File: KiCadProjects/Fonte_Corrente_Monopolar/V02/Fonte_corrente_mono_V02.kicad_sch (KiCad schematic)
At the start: 33 parts, among them J1 alimentacao analogica, J2 sinais analogicos, J3 comunicacao / sinais digitais, J4 signal select, J7 +3.3V | +5.0V, U1-howland1 AD828AN, U2-INA-I1 INA128, U3-cond1 AD828AN

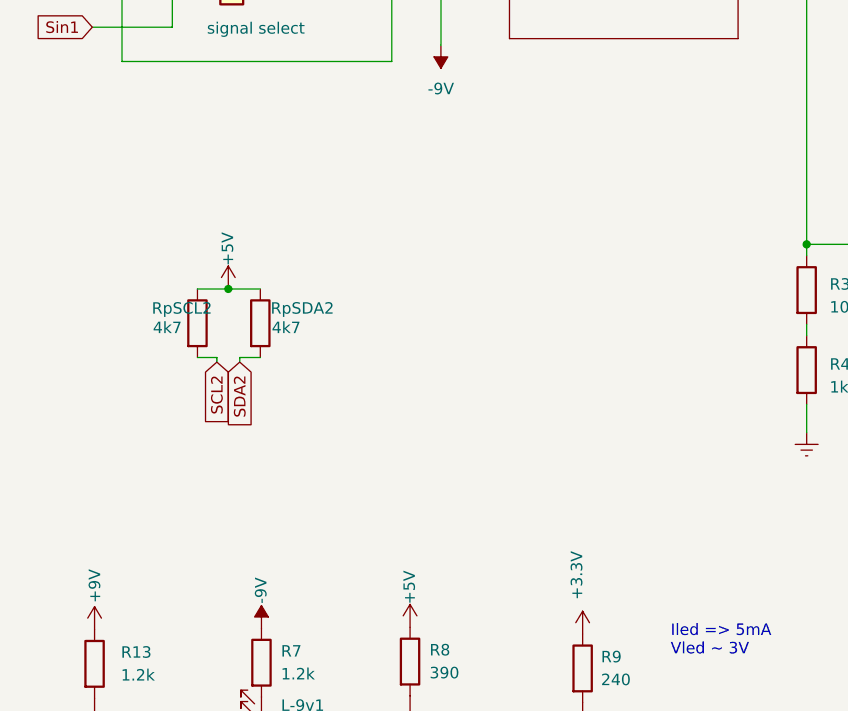
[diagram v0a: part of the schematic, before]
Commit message: temp
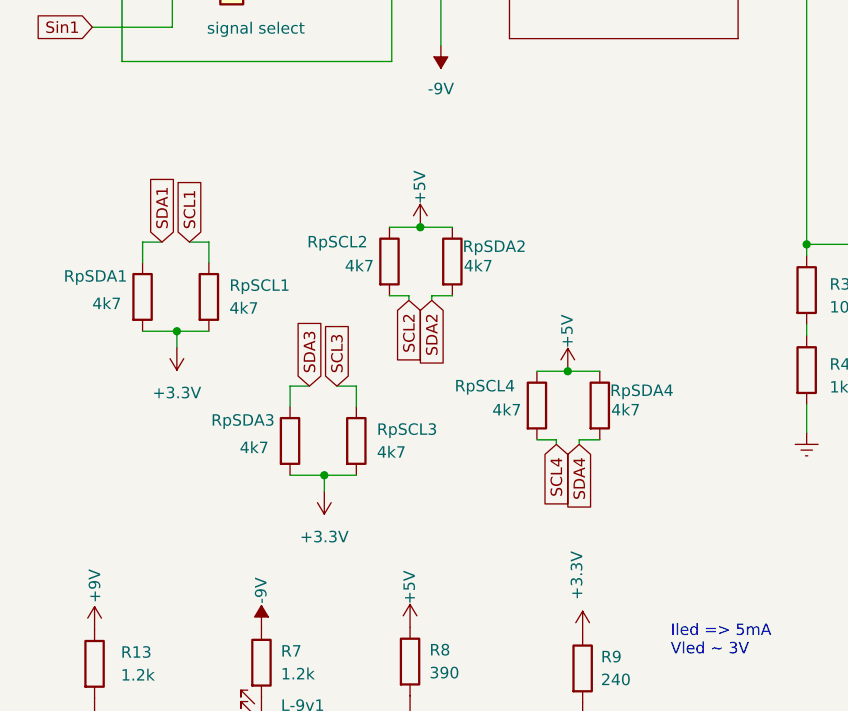
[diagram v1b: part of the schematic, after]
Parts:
- added RpSCL1, RpSCL3, RpSCL4, RpSDA1, RpSDA3, RpSDA4: 4k7, Resistor_THT:R_Axial_DIN0207_L6.3mm_D2.5mm_P7.62mm_Horizontal, symbol Device:R
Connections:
- net +3.3V: now also RpSCL1.2, RpSCL3.2, RpSDA1.2, RpSDA3.2
- net +5V: now also RpSCL4.1, RpSDA4.1
- net SCL1: now also RpSCL1.1
- net SCL3: now also RpSCL3.1
- net SCL4: now also RpSCL4.2
- net SDA1: now also RpSDA1.1
- net SDA3: now also RpSDA3.1
- net SDA4: now also RpSDA4.2
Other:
- moved on the sheet: RpSCL2, RpSDA2
